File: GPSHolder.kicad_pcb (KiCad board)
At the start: 2 copper layers, 29.5 x 38.1 mm, 7 parts, among them J1 TEST_1P, J2 TEST_1P, J3 TEST_1P, J4 TEST_1P

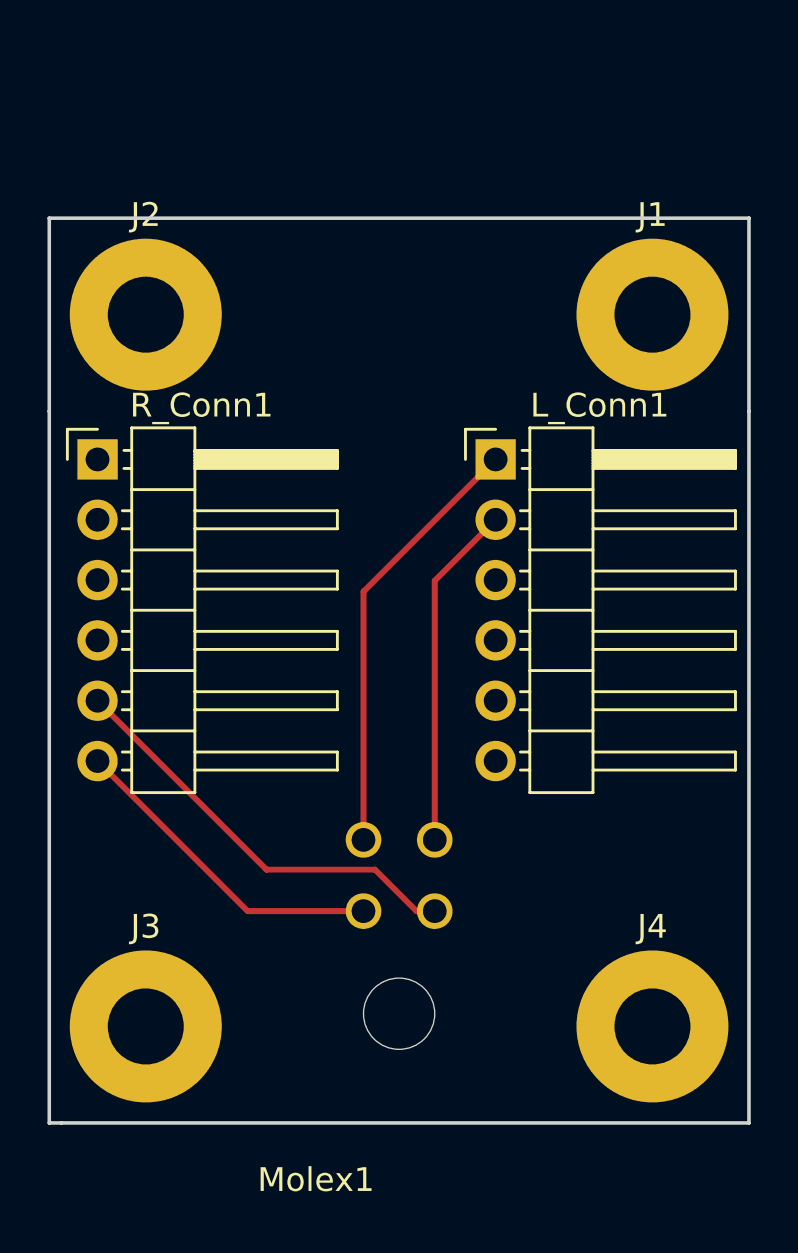
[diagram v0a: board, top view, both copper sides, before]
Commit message: Add files via upload
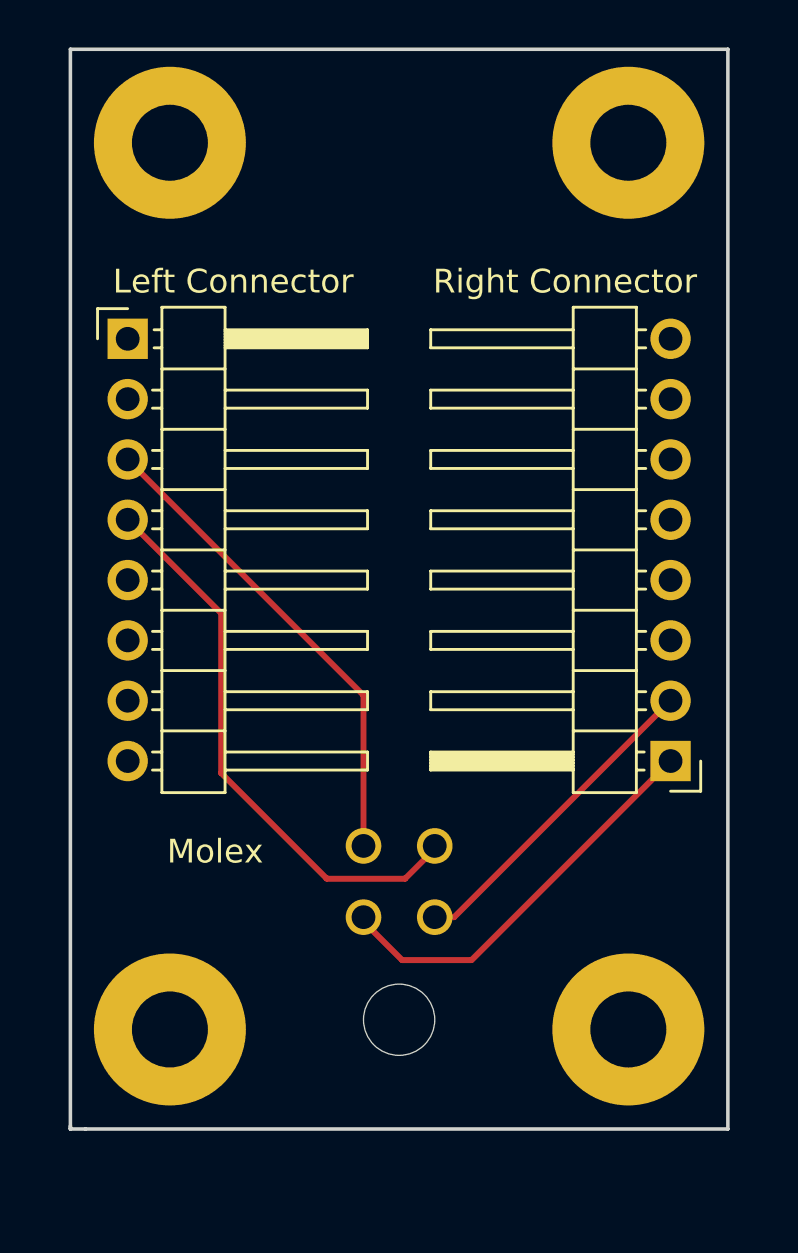
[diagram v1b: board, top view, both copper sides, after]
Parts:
- removed L_Conn1, R_Conn1: Conn_01x06_Male, Pin_Headers:Pin_Header_Angled_1x06_Pitch2.54mm
- added Left Connector: Conn_01x08_Male, Pin_Headers:Pin_Header_Angled_1x08_Pitch2.54mm, F.Cu at (137.9, 90.9)
- added Right Connector: Conn_01x08_Male, Pin_Headers:Pin_Header_Angled_1x08_Pitch2.54mm, F.Cu at (160.8, 108.7)
- moved J1 7.31 mm to (159.0, 82.7)
- moved J2 7.31 mm to (139.7, 82.7)
- moved J4 1.02 mm to (159.0, 120.0)
- moved J3 1.02 mm to (139.7, 120.0)
- moved Molex 0.25 mm to (149.4, 124.2)
- renumbered Molex1 to Molex
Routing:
- net Net-(L_Conn1-Pad4): track 14.5 -> 23.8 mm
- net Net-(Molex1-Pad1): track 17.9 -> 13.7 mm
- net Net-(Molex1-Pad2): track 13.8 -> 17.5 mm
- net Net-(L_Conn1-Pad3): track 18.3 -> 20.4 mm
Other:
- board size 29.5 x 38.1 mm -> 27.7 x 45.5 mm
